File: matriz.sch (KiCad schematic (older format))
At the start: 69 parts

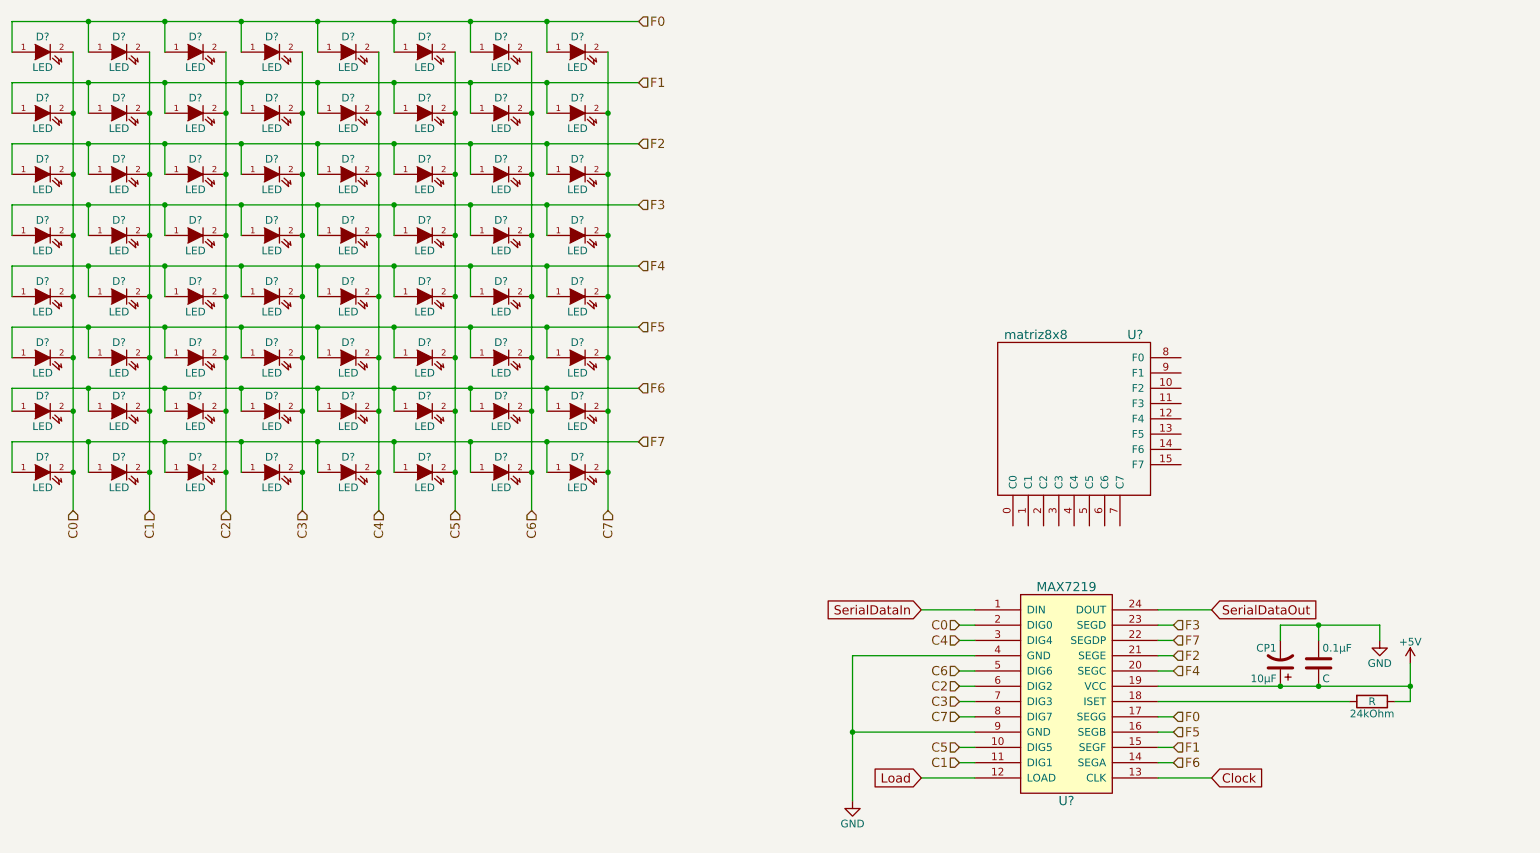
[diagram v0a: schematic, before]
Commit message: hola soy un commit hecho por nahuel 	# with '#' will be ignored, and an empty message aborts the commit. 	#
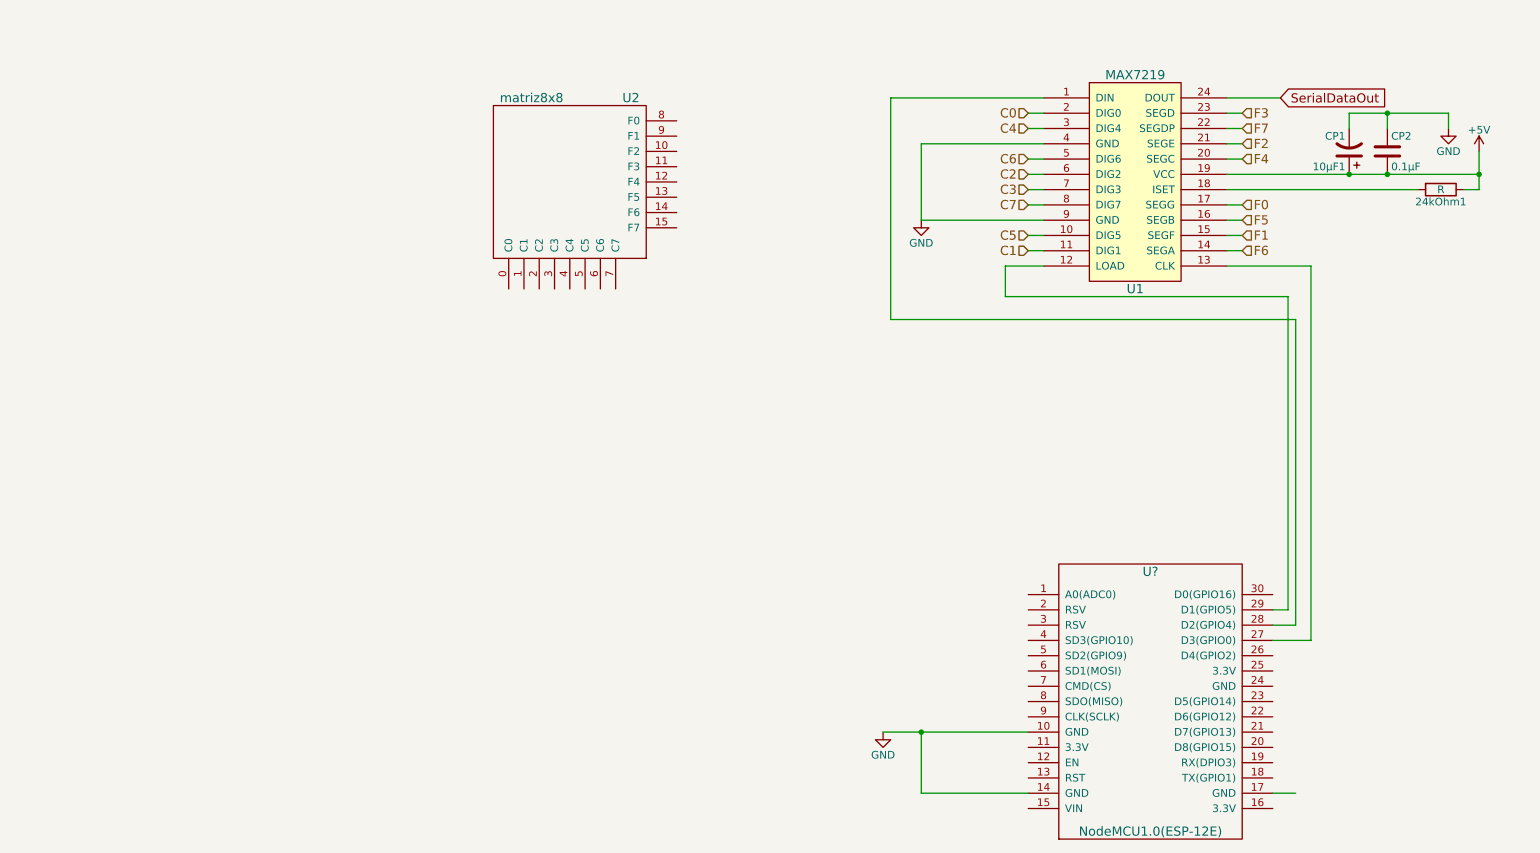
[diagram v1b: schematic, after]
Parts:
- removed D? (x64): LED, symbol LED
- added U?: NodeMCU1.0(ESP-12E), symbol NodeMCU1.0(ESP-12E)
- CP2: renamed from 0.1µF; value C -> 0.1µF
- gave numbers to parts that had none: 2
- renumbered 10µF to 10µF1, 24kOhm to 24kOhm1
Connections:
- net GND: now also U?.10 (GND), U?.14 (GND)
- net Clock: no longer names the net of U1.13 (CLK)
- net Clock: now also U?.27 (D3(GPIO0))
- net Load: no longer names the net of U1.12 (LOAD)
- net Load: now also U?.29 (D1(GPIO5))
- net SerialDataIn: no longer names the net of U1.1 (DIN)
- net SerialDataIn: now also U?.28 (D2(GPIO4))
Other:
- moved on the sheet: 10µF1, 24kOhm1, CP2, U1, U2

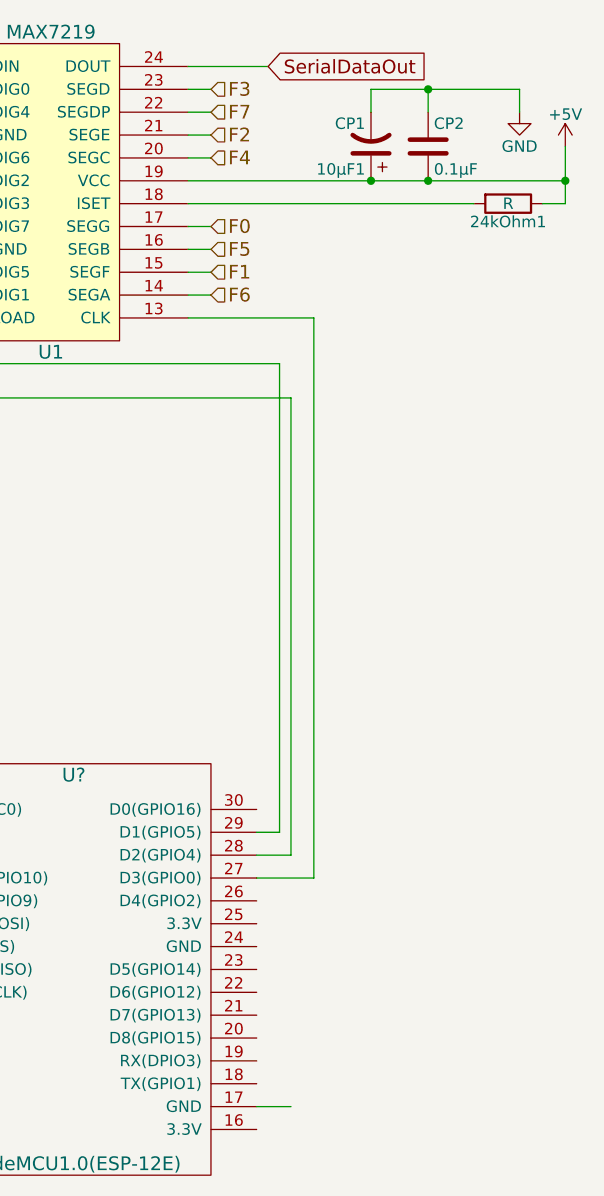
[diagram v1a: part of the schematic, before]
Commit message: Cosas
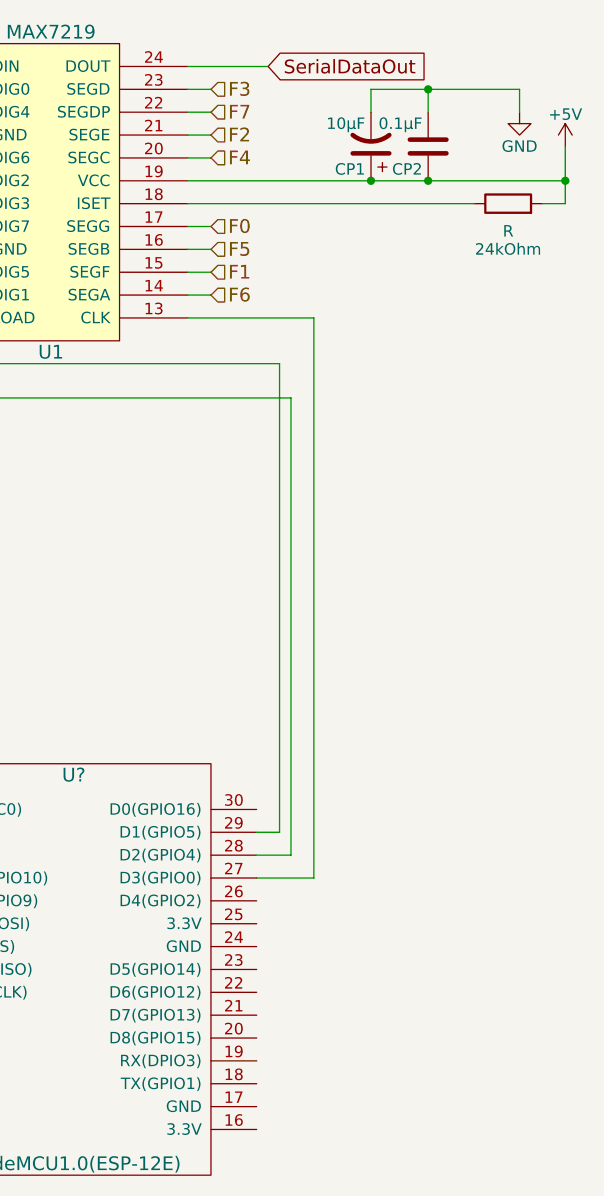
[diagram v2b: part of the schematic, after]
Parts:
- removed 10µF1: CP1, symbol CP1
- removed 24kOhm1: R, symbol R
- added CP1: 10µF, symbol CP1
- added R: 24kOhm, symbol R
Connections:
- net +5V: now also CP2.1, CP1.1, R.2; no longer CP2.2
- net GND: now also CP2.2, CP1.2; no longer CP2.1
- net at U1.18 (ISET): now also R.1
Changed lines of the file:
@@
 EESchema Schematic File Version 2
+LIBS:power
+LIBS:device
+LIBS:switches
+LIBS:relays
+LIBS:motors
+LIBS:transistors
+LIBS:conn
+LIBS:linear
+LIBS:regul
+LIBS:74xx
+LIBS:cmos4000
+LIBS:adc-dac
+LIBS:memory
+LIBS:xilinx
+LIBS:microcontrollers
+LIBS:dsp
+LIBS:microchip
+LIBS:analog_switches
+LIBS:motorola
+LIBS:texas
+LIBS:intel
+LIBS:audio
+LIBS:interface
+LIBS:digital-audio
+LIBS:philips
+LIBS:display
+LIBS:cypress
+LIBS:siliconi
+LIBS:opto
+LIBS:atmel
+LIBS:contrib
+LIBS:valves
 LIBS:max
 LIBS:leds
 LIBS:matriz8x8
-LIBS:power
-LIBS:device
 LIBS:wemosD1
 LIBS:ESP8266
@@
 $EndComp
 $Comp
-L C CP2
-U 1 1 59C7ECB1
-P 9750 1800
-F 0 "CP2" H 9775 1900 50  0000 L CNN
-F 1 "0.1µF" H 9775 1700 50  0000 L CNN
-F 2 "" H 9788 1650 50  0001 C CNN
-F 3 "" H 9750 1800 50  0001 C CNN
-	1    9750 1800
-	1    0    0    -1
-$EndComp
-$Comp
 L GND #PWR03
 U 1 1 59C7F084
@@
 	1    10150 1650
 	1    0    0    -1
-$EndComp
-$Comp
-L R 24kOhm1
-U 1 1 59C803C2
-P 10100 2050
-F 0 "24kOhm1" V 10180 2050 50  0000 C CNN
-F 1 "R" V 10100 2050 50  0000 C CNN
-F 2 "" V 10030 2050 50  0001 C CNN
-F 3 "" H 10100 2050 50  0001 C CNN
-	1    10100 2050
-	0    1    1    0
 $EndComp
 Text GLabel 9050 1450 2    60   Input ~ 0
@@
 Text HLabel 7400 2350 0    60   Input ~ 0
 C5
-$Comp
-L CP1 10µF1
-U 1 1 59E154D8
-P 9500 1800
-F 0 "10µF1" H 9525 1900 50  0000 L CNN
-F 1 "CP1" H 9525 1700 50  0000 L CNN
-F 2 "" H 9500 1800 50  0001 C CNN
-F 3 "" H 9500 1800 50  0001 C CNN
-	1    9500 1800
-	-1   0    0    1
-$EndComp
 Text HLabel 7400 2150 0    60   Input ~ 0
 C7
@@
 	8700 2150 8800 2150
 Wire Wire Line
-	8800 1850 8700 1850
-Wire Wire Line
-	8800 1750 8700 1750
-Wire Wire Line
-	8800 1650 8700 1650
-Wire Wire Line
 	8700 2550 9250 2550
-Wire Wire Line
-	8800 1550 8700 1550
 Wire Wire Line
 	7500 2350 7400 2350
@@
 $EndComp
 Wire Wire Line
-	9000 6000 9150 6000
-Wire Wire Line
 	6700 1750 6700 2250
 Wire Wire Line
@@
 	1    0    0    -1
 $EndComp
+$Comp
+L C CP2
+U 1 1 59FFA831
+P 9750 1800
+F 0 "CP2" H 9775 1900 50  0000 L CNN
+F 1 "0.1µF" H 9775 1700 50  0000 L CNN
+F 2 "" H 9788 1650 50  0001 C CNN
+F 3 "" H 9750 1800 50  0001 C CNN
+	1    9750 1800
+	-1   0    0    1
+$EndComp
+$Comp
+L CP1 CP1
+U 1 1 59FFA866
+P 9500 1800
+F 0 "CP1" H 9525 1900 50  0000 L CNN
+F 1 "10µF" H 9525 1700 50  0000 L CNN
+F 2 "" H 9500 1800 50  0001 C CNN
+F 3 "" H 9500 1800 50  0001 C CNN
+	1    9500 1800
+	-1   0    0    1
+$EndComp
+$Comp
+L R R
+U 1 1 59FFAE64
+P 10100 2050
+F 0 "R" V 9950 2050 50  0000 C TNN
+F 1 "24kOhm" V 9900 2050 50  0000 C CNN
+F 2 "" V 10030 2050 50  0001 C CNN
+F 3 "" H 10100 2050 50  0001 C CNN
+	1    10100 2050
+	0    -1   -1   0
+$EndComp
+Wire Wire Line
+	8800 1550 8700 1550
+Wire Wire Line
+	8800 1650 8700 1650
+Wire Wire Line
+	8800 1750 8700 1750
+Wire Wire Line
+	8800 1850 8700 1850
 $EndSCHEMATC

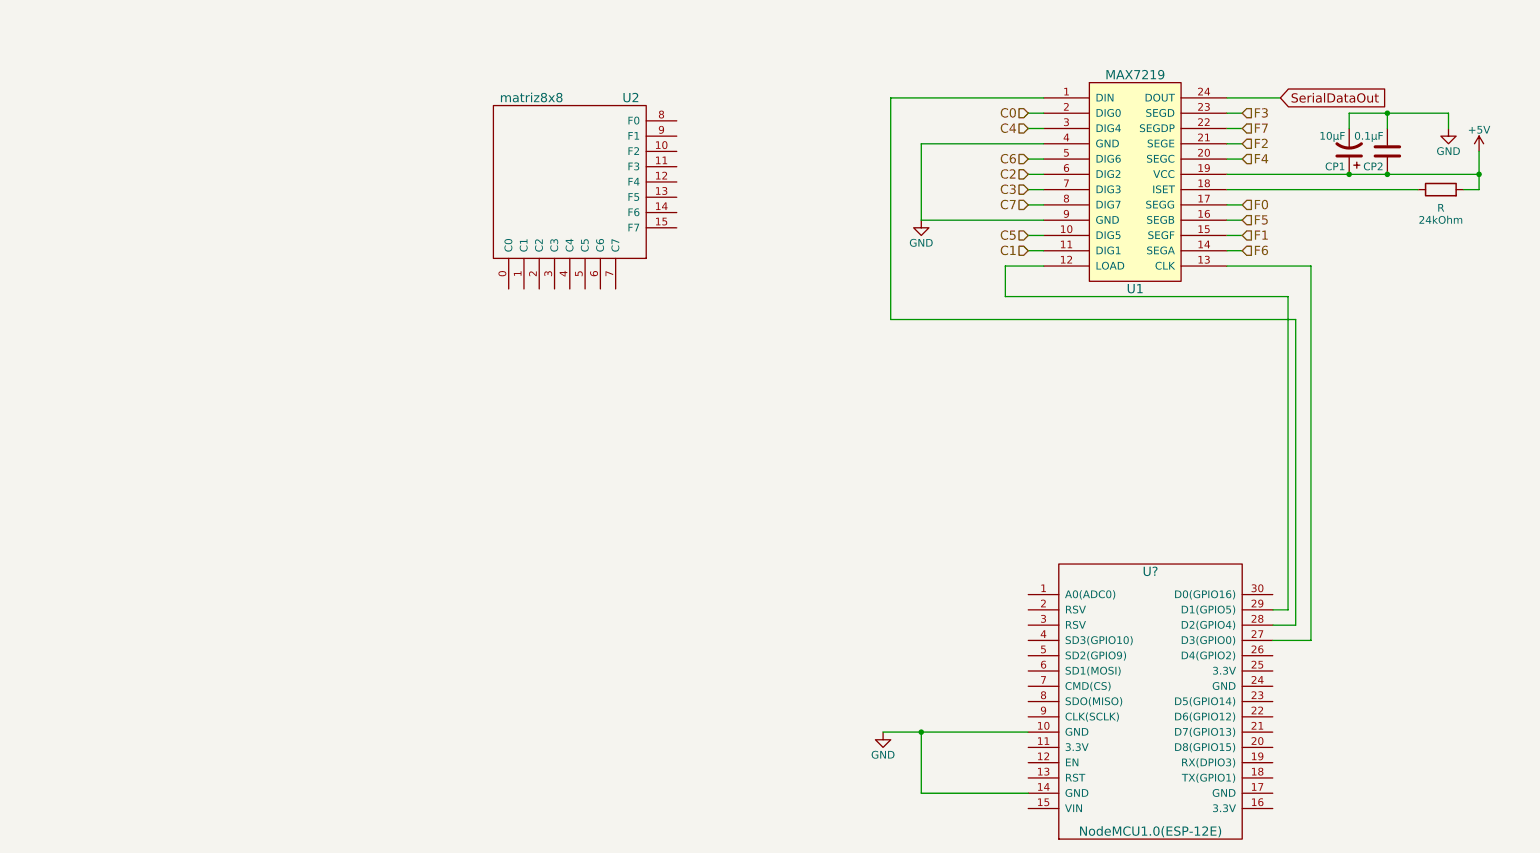
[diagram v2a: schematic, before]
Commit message: Sin labels y mas
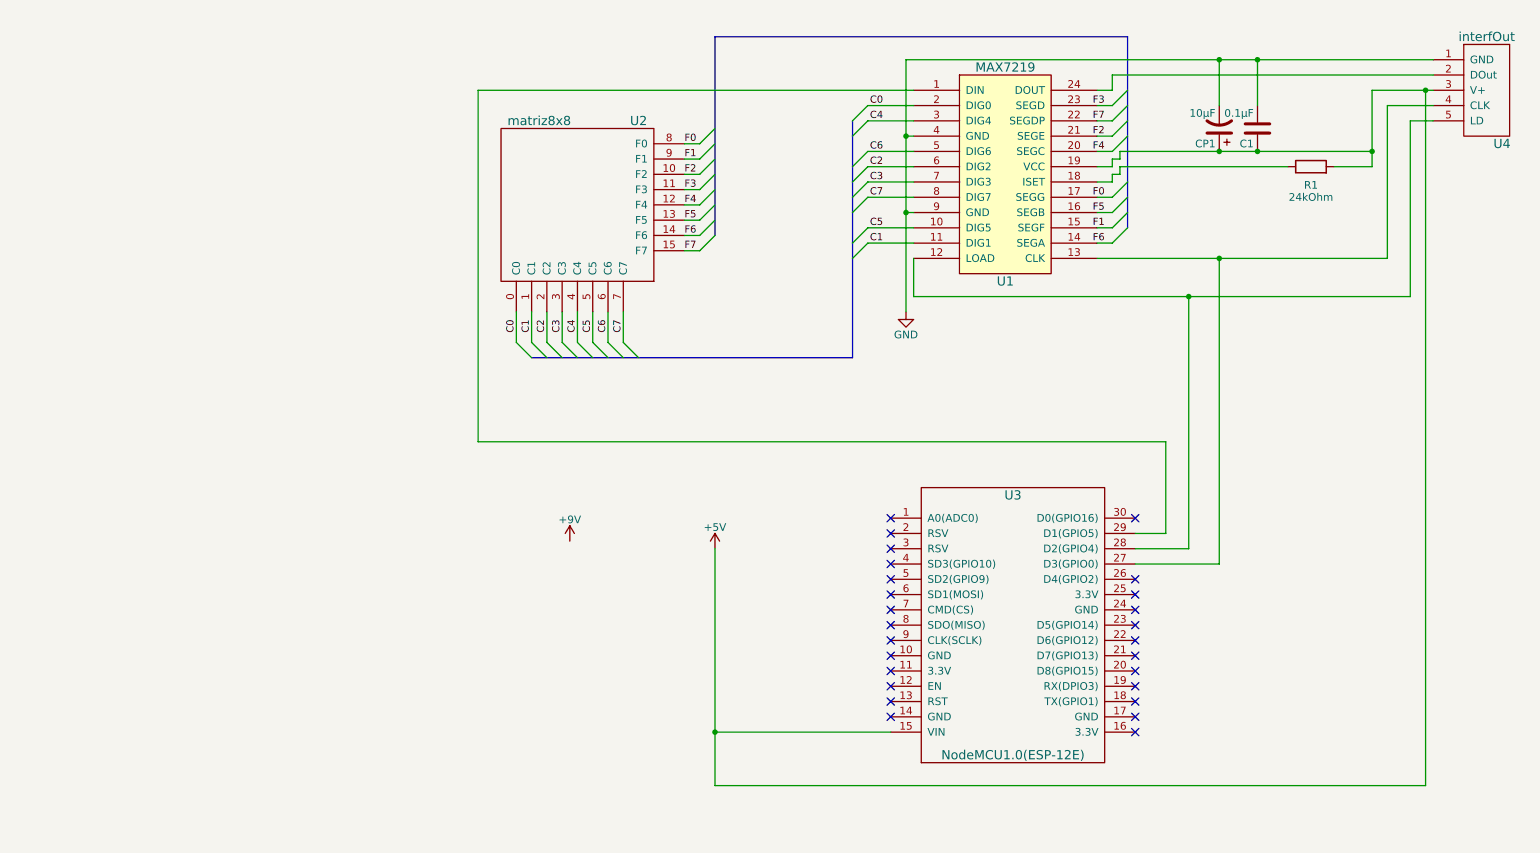
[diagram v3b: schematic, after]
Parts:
- added U4: interfOut, symbol interfOut
- gave numbers to parts that had none: 1
- renumbered CP2 to C1, R to R1
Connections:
- net +5V: now also U3.15 (VIN), U4.3 (V+)
- net C0: now also U2.0 (C0)
- net C1: now also U2.1 (C1)
- net C2: now also U2.2 (C2)
- net C3: now also U2.3 (C3)
- net C4: now also U2.4 (C4)
- net C5: now also U2.5 (C5)
- net C6: now also U2.6 (C6)
- net C7: now also U2.7 (C7)
- net F0: now also U2.8 (F0)
- net F1: now also U2.9 (F1)
- net F2: now also U2.10 (F2)
- net F3: now also U2.11 (F3)
- net F4: now also U2.12 (F4)
- net F5: now also U2.13 (F5)
- net F6: now also U2.14 (F6)
- net F7: now also U2.15 (F7)
- net GND: now also U4.1 (GND); no longer U3.10 (GND), U3.14 (GND)
- net at U1.1 (DIN): now also U3.29 (D1(GPIO5)); no longer U3.28 (D2(GPIO4))
- net at U1.12 (LOAD): now also U3.28 (D2(GPIO4)), U4.5 (LD); no longer U3.29 (D1(GPIO5))
- net at U1.13 (CLK), U3.27 (D3(GPIO0)): now also U4.4 (CLK)
- net SerialDataOut: no longer names the net of U1.24 (DOUT)
- net SerialDataOut: now also U4.2 (DOut)
- no-connect marks 0 -> 26
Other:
- moved on the sheet: C1, CP1, R1, U1, U3
